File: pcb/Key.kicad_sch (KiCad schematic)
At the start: 4 parts, among them U4 TMR2652D

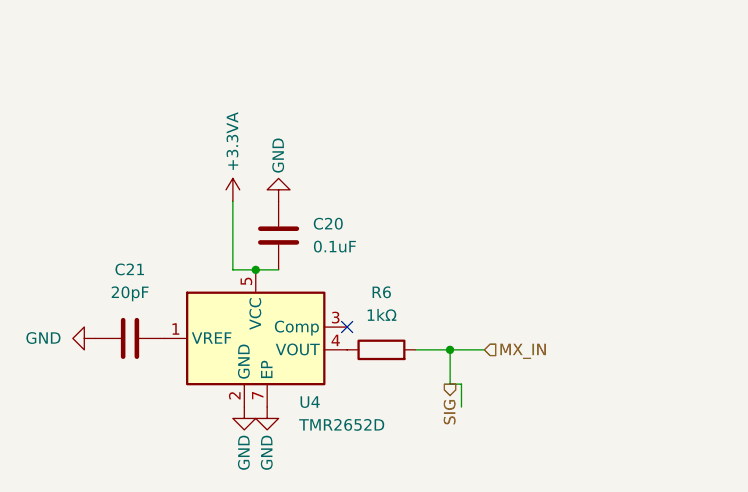
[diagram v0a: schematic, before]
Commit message: feat: working changes
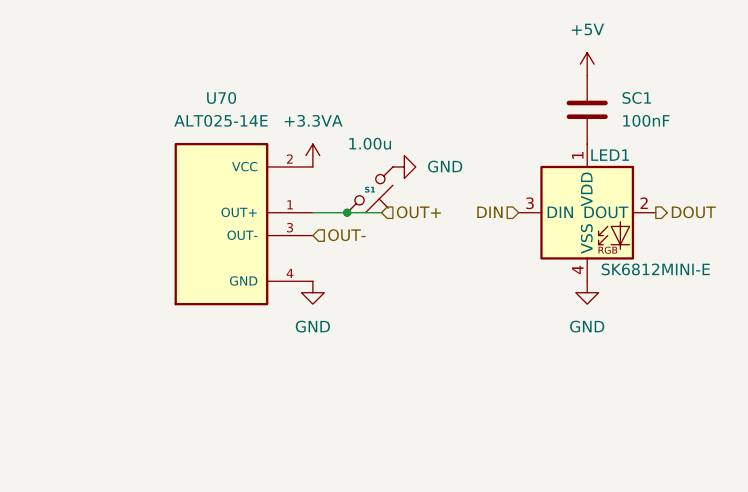
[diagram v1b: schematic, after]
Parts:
- removed C20: 0.1uF, Capacitor_SMD:C_0402_1005Metric, symbol Device:C
- removed C21: 20pF, Capacitor_SMD:C_0402_1005Metric, symbol Device:C
- removed R6: 1kΩ, Resistor_SMD:R_0402_1005Metric, symbol Device:R
- removed U4: TMR2652D, prometheus-65-footprints:TMR2652D, symbol prometheus-65-symbols:TMR2652D
- added LED1: SK6812MINI-E, PCM_marbastlib-various:LED_6028R, symbol PCM_marbastlib-various:SK6812MINI-E
- added S1: 1.00u, ScottoKeebs_Hotswap:Hotswap_MX_Plated_1.00u, symbol ScottoKeebs:Placeholder_Keyswitch
- added SC1: 100nF, Capacitor_SMD:C_0402_1005Metric, symbol Device:C
- added U70: ALT025-14E, prometheus-65-footprints:ALT025-14E, symbol prometheus-65-symbols:ALT025-14E
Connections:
- net +3.3VA: now also U70.2 (VCC)
- net GND: now also LED1.4 (VSS), S1.2, U70.4 (GND)
- new net: LED1.1 (VDD), SC1.2
- new net +5V: SC1.1
- new net DIN: LED1.3 (DIN)
- new net DOUT: LED1.2 (DOUT)
- new net OUT+: S1.1, U70.1 (OUT+)
- new net OUT-: U70.3 (OUT-)
- no-connect marks 1 -> 0
